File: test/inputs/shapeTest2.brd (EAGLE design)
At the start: 2 parts

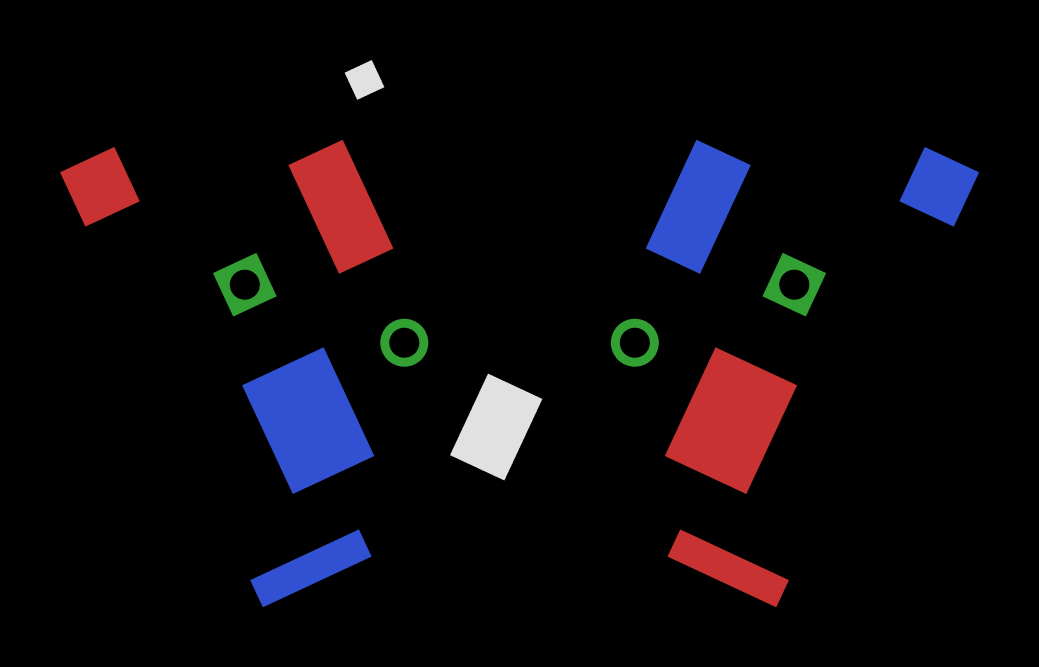
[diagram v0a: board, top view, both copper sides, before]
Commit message: Improved tests
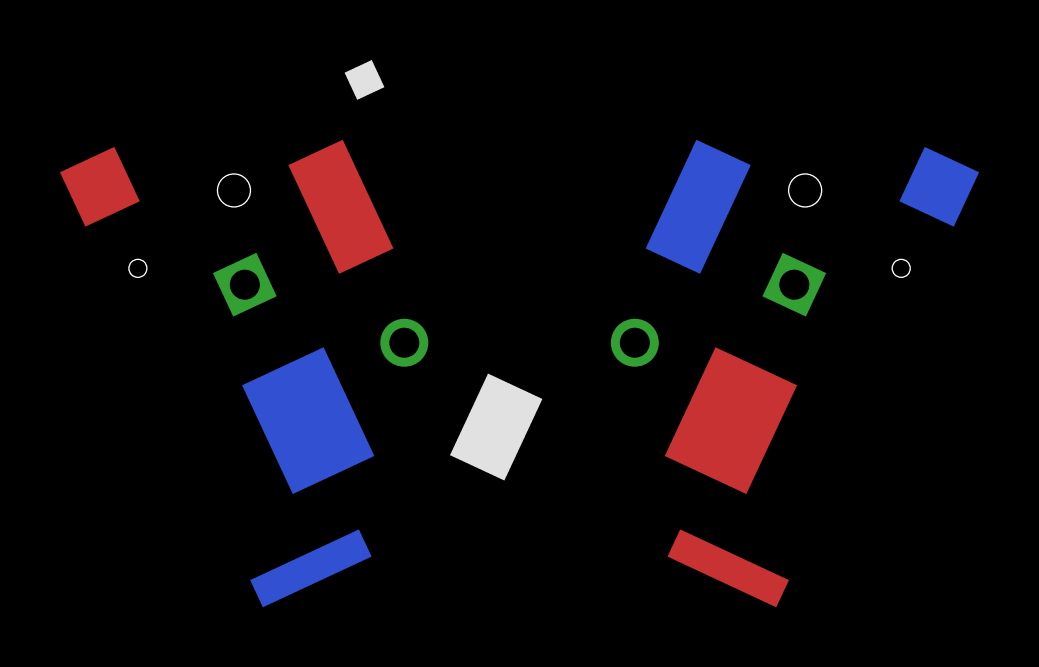
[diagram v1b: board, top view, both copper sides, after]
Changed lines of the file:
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@@
 <layer number="97" name="Info" color="7" fill="1" visible="no" active="no"/>
 <layer number="98" name="Guide" color="6" fill="1" visible="no" active="no"/>
-<layer number="101" name="tTest2" color="13" fill="1" visible="yes" active="yes"/>
-<layer number="102" name="bTest2" color="14" fill="1" visible="yes" active="yes"/>
+<layer number="102" name="onBoard" color="10" fill="3" visible="yes" active="yes"/>
+<layer number="103" name="offBoard" color="9" fill="3" visible="yes" active="yes"/>
+<layer number="151" name="tTest2" color="13" fill="1" visible="yes" active="yes"/>
+<layer number="152" name="bTest2" color="14" fill="1" visible="yes" active="yes"/>
 </layers>
 <board>
